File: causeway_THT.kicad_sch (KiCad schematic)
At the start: 161 parts, among them J1 12402054M611A, SW1 SW_Cherry_MX_PCB_1.50u, SW10 SW_Cherry_MX_1.00u_PCB, SW11 SW_Cherry_MX_1.00u_PCB, SW12 SW_Cherry_MX_1.00u_PCB, SW13 SW_Cherry_MX_1.00u_PCB, SW14 SW_Cherry_MX_PCB_1.50u, SW15 SW_Cherry_MX_PCB_1.50u, SW16 SW_Cherry_MX_1.00u_PCB, SW17 SW_Cherry_MX_1.00u_PCB, SW18 SW_Cherry_MX_1.00u_PCB, SW19 SW_Cherry_MX_1.00u_PCB, SW2 SW_Cherry_MX_1.00u_PCB, SW20 SW_Cherry_MX_1.00u_PCB, SW21 SW_Cherry_MX_1.00u_PCB, SW22 SW_Cherry_MX_1.00u_PCB, SW23 SW_Cherry_MX_1.00u_PCB, SW24 SW_Cherry_MX_1.00u_PCB, SW25 SW_Cherry_MX_1.00u_PCB, SW26 SW_Cherry_MX_1.00u_PCB, SW27 SW_Cherry_MX_1.00u_PCB, SW28 SW_Cherry_MX_PCB_1.50u, SW29 SW_Cherry_MX_1.00u_PCB, SW3 SW_Cherry_MX_1.00u_PCB, SW30 SW_Cherry_MX_1.00u_PCB, SW31 SW_Cherry_MX_1.00u_PCB, SW32 SW_Cherry_MX_1.00u_PCB, SW33 SW_Cherry_MX_1.00u_PCB, SW34 SW_Cherry_MX_1.00u_PCB, SW35 SW_Cherry_MX_1.00u_PCB, SW36 SW_Cherry_MX_1.00u_PCB, SW37 SW_Cherry_MX_1.00u_PCB, SW38 SW_Cherry_MX_1.00u_PCB, SW39 SW_Cherry_MX_1.00u_PCB, SW4 SW_Cherry_MX_1.00u_PCB, SW40 SW_Cherry_MX_1.00u_PCB, SW41 SW_Cherry_MX_PCB_1.50u, SW42 SW_Cherry_MX_PCB_1.50u, SW43 SW_Cherry_MX_PCB_1.50u, SW44 SW_Cherry_MX_1.00u_PCB, SW45 SW_Cherry_MX_1.00u_PCB, SW46 SW_Cherry_MX_1.00u_PCB, SW47 SW_Cherry_MX_1.00u_PCB, SW48 SW_Cherry_MX_1.00u_PCB, SW49 SW_Cherry_MX_1.00u_PCB, SW5 SW_Cherry_MX_1.00u_PCB, SW50 SW_Cherry_MX_1.00u_PCB, SW51 SW_Cherry_MX_1.00u_PCB, SW52 SW_Cherry_MX_1.00u_PCB, SW53 SW_Cherry_MX_1.00u_PCB, SW54 SW_Cherry_MX_1.00u_PCB, SW55 SW_Cherry_MX_1.00u_PCB, SW56 SW_Cherry_MX_PCB_1.50u, SW57 SW_Cherry_MX_PCB_1.50u, SW58 SW_Cherry_MX_1.00u_PCB, SW59 SW_Cherry_MX_1.00u_PCB, SW6 SW_Cherry_MX_1.00u_PCB, SW60 SW_Cherry_MX_1.00u_PCB, SW61 SW_Cherry_MX_PCB_3.00u, SW62 SW_Cherry_MX_PCB_3.00u, SW63 SW_Cherry_MX_1.00u_PCB, SW64 SW_Cherry_MX_1.00u_PCB, SW65 SW_Cherry_MX_1.00u_PCB, SW66 SW_Cherry_MX_PCB_1.50u, SW67 SW_Cherry_MX_PCB_1.50u_90deg, SW68 SW_Cherry_MX_PCB_1.50u_90deg, SW69 SW_Cherry_MX_PCB_1.50u_90deg, SW7 SW_Cherry_MX_1.00u_PCB, SW70 SW_Cherry_MX_PCB_1.50u_90deg, SW71 SW_Cherry_MX_PCB_3.00u, SW72 SW_Cherry_MX_PCB_3.00u, SW8 SW_Cherry_MX_1.00u_PCB, SW9 SW_Cherry_MX_1.00u_PCB, U1 ATmega32A-P, Y1 16MHz

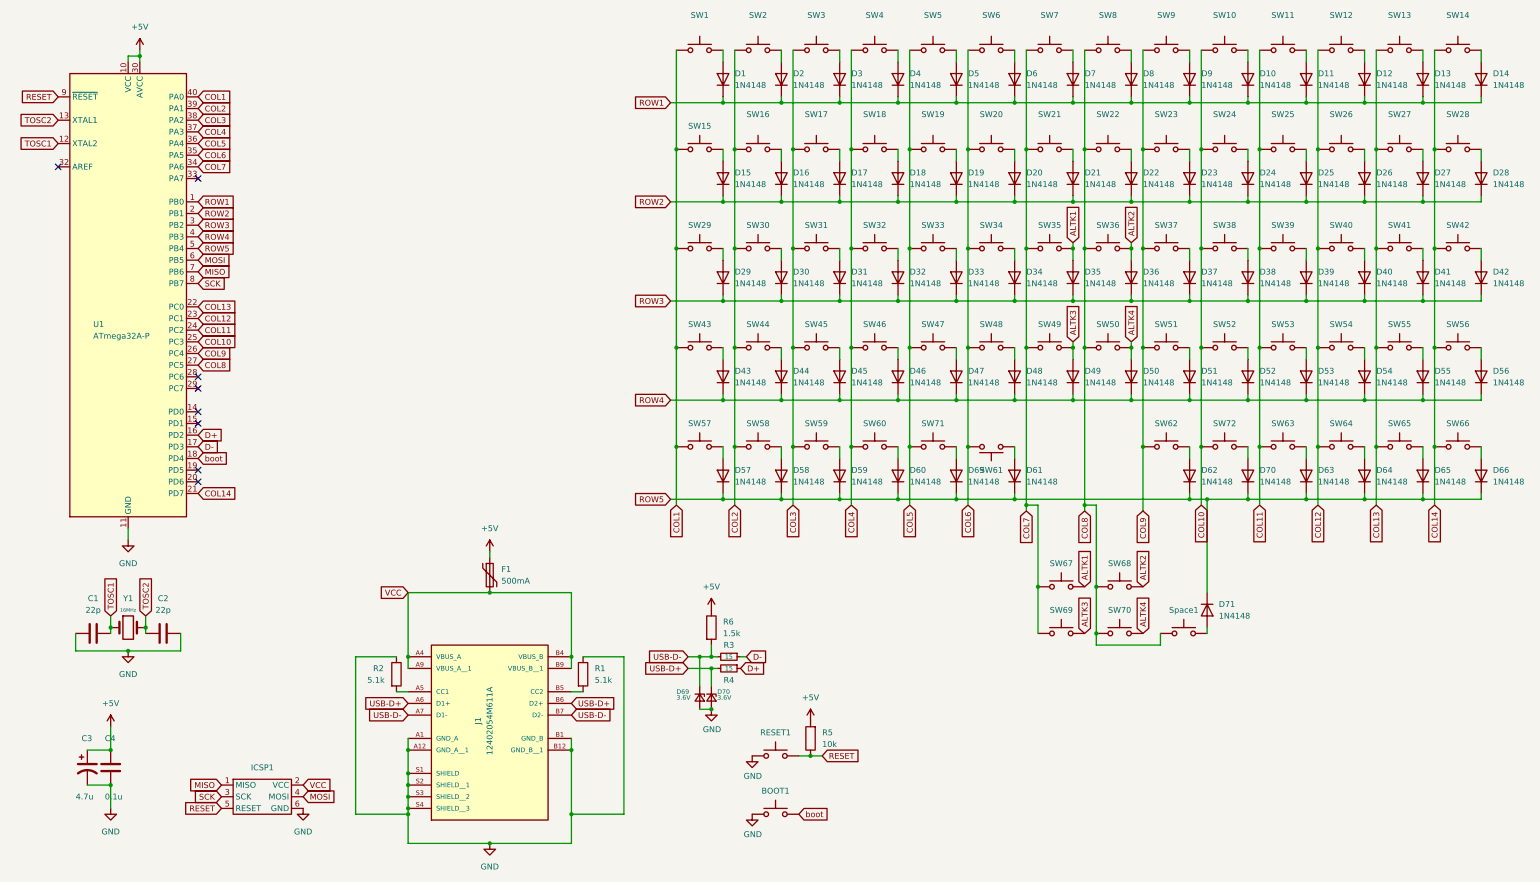
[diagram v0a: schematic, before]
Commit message: labeling
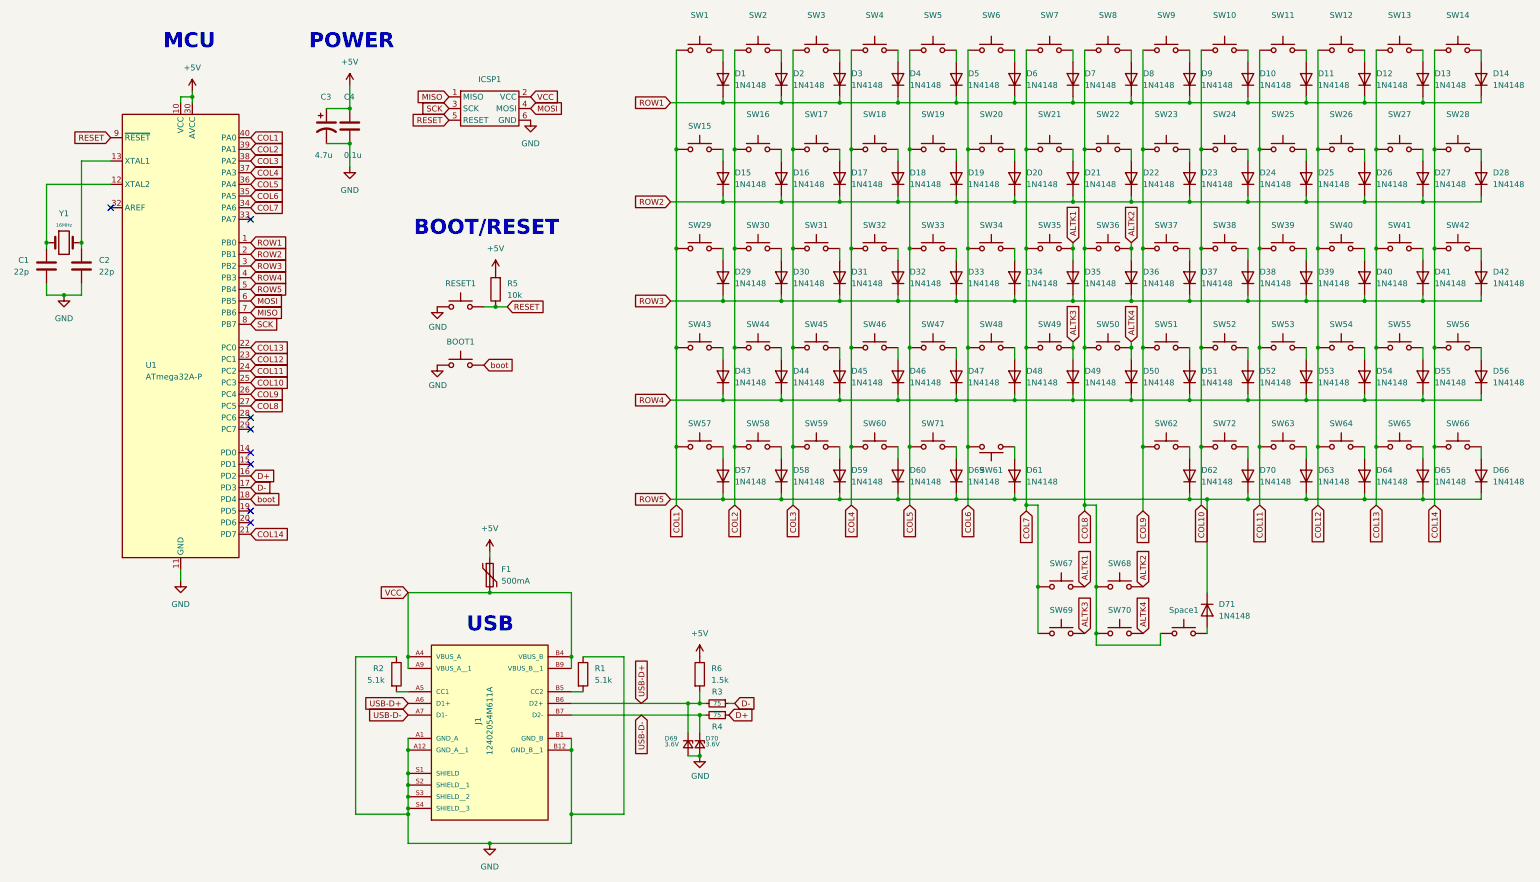
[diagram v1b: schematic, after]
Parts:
- R3, R4: value 15 -> 75
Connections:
- net GND: now also C1.2, C2.1; no longer C1.1, C2.2
- net USB-D+: now also D69.1 (K), R3.2, R6.2; no longer D70.1 (K), R4.2
- net USB-D-: now also D70.1 (K), R4.2; no longer D69.1 (K), R3.2, R6.2
- net TOSC1: no longer names the net of U1.12 (XTAL2), Y1.1
- net TOSC1: now also C1.1; no longer C1.2
- net TOSC2: no longer names the net of U1.13 (XTAL1), Y1.2
- net TOSC2: now also C2.2; no longer C2.1
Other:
- note added: "BOOT/RESET"
- note added: "MCU"
- note added: "POWER"
- note added: "USB"
- moved on the sheet: BOOT1, C1, C2, C3, C4, D69, D70, ICSP1, R3, R4, R5, R6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

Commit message: Update causeway_THT.kicad_sch
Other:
- company: (none) -> iSandRocks
- title: (none) -> Causeway_THT
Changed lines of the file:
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@@
 (kicad_sch (version 20230121) (generator eeschema)
   (paper "USLegal")
+  (title_block
+    (title "Causeway_THT")
+    (date "2024-02-06")
+    (company "iSandRocks")
+  )
   (junction (at 205.74 33.02) (diameter 0) (color 0 0 0 0)
   )
